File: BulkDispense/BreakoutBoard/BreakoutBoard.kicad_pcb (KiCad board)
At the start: 2 copper layers, 74.5 x 119 mm, 36 parts, among them J1 BS1, J10 OS3, J11 OS4, J12 FS1, J13 FS3, J14 PCV, J15 FS2, J16 FS4, J17 WL1, J18 WL2, J19 Analog Inputs, J2 BS2, J20 R0~R3, J21 R4~R7, J22 R8~R9, J23 Digital IN + R0~R4, J24 WB1, J25 WB2, J26 Digital Outputs, J27 R4~R9, J28 WV1, J29 WV2, J3 OS1, J30 Flow Sensors (PORT2), J4 OS2, J5 PS, J6 MV1&2, J7 MV3&4, J8 BS3, J9 BS4

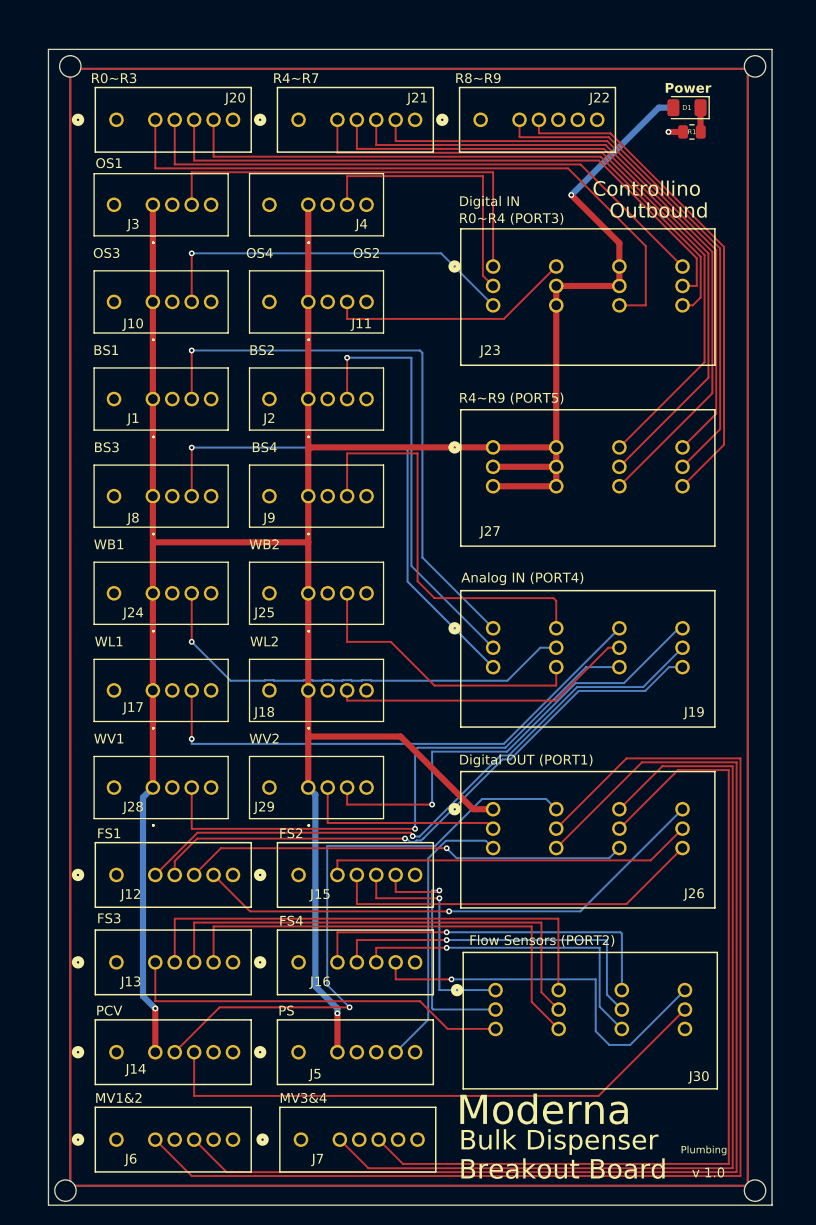
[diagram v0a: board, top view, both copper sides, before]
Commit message: Design Overhaul
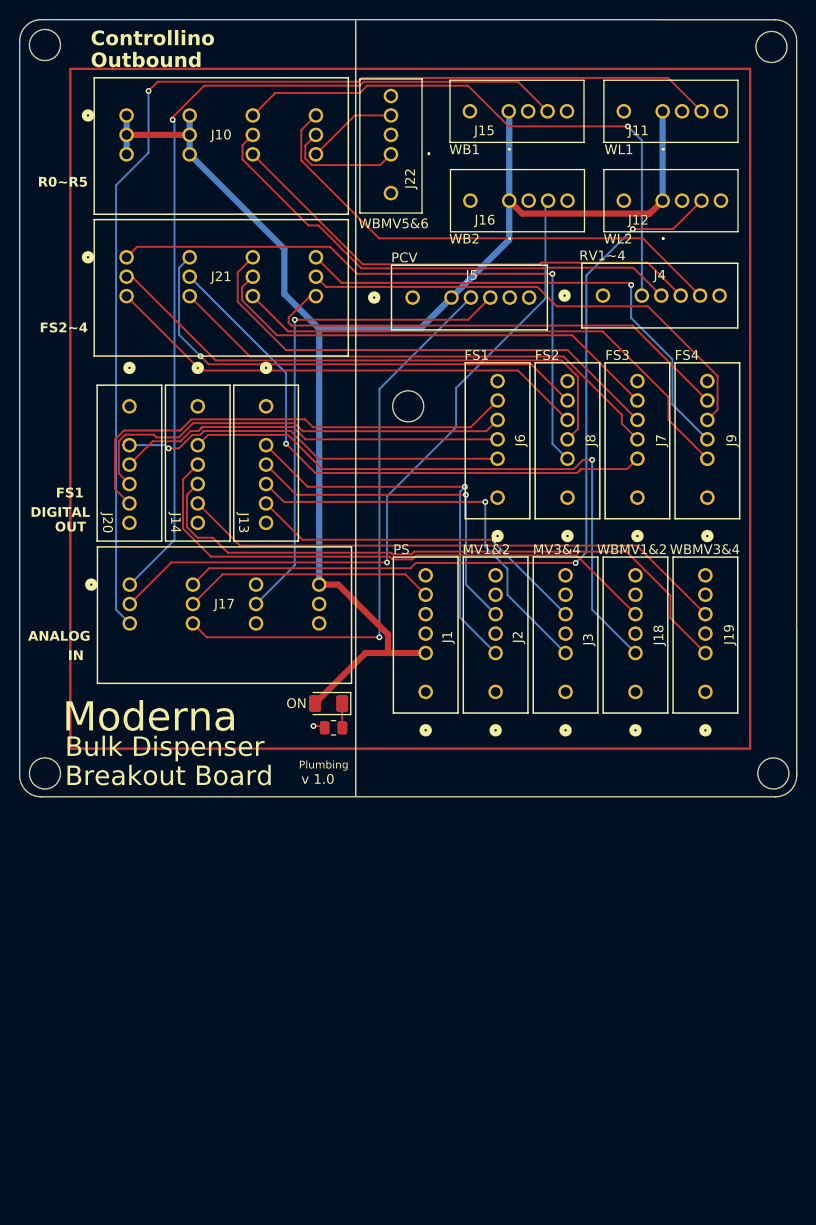
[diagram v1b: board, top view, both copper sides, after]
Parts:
- removed J23: Digital IN + R0~R4, PartsLibrary:CONN_37212-62M3-003PL_3MM
- removed J24: WB1, PartsLibrary:3720362A3003PL
- removed J25: WB2, PartsLibrary:3720362A3003PL
- removed J26: Digital Outputs, PartsLibrary:CONN_37212-62M3-003PL_3MM
- removed J27: R4~R9, PartsLibrary:CONN_37212-62M3-003PL_3MM
- removed J28: WV1, PartsLibrary:3720362A3003PL
- removed J29: WV2, PartsLibrary:3720362A3003PL
- removed J30: Flow Sensors (PORT2), PartsLibrary:CONN_37212-62M3-003PL_3MM
- added H5: MountingHole, MountingHole:MountingHole_3.2mm_M3, F.Cu at (181.8, 106.8)
- H1, H2, H3, H4: footprint MountingHole:MountingHole_2.2mm_M2 -> MountingHole:MountingHole_3.2mm_M3
- J1: value BS1 -> PS; footprint PartsLibrary:3720362A3003PL -> PartsLibrary:CONN_37204-62A3-004PL_3MM
- J10: value OS3 -> R0~R5; footprint PartsLibrary:3720362A3003PL -> PartsLibrary:CONN_37212-62M3-003PL_3MM
- J11: value OS4 -> WL1
- J12: value FS1 -> WL2; footprint PartsLibrary:CONN_37204-62A3-004PL_3MM -> PartsLibrary:3720362A3003PL
- J13: value FS3 -> DigitalOUT 0~3
- J14: value PCV -> DigitalOUT 4~7
- J15: value FS2 -> WB1; footprint PartsLibrary:CONN_37204-62A3-004PL_3MM -> PartsLibrary:3720362A3003PL
- J16: value FS4 -> WB2; footprint PartsLibrary:CONN_37204-62A3-004PL_3MM -> PartsLibrary:3720362A3003PL
- J17: value WL1 -> AnalogIOs; footprint PartsLibrary:3720362A3003PL -> PartsLibrary:CONN_37212-62M3-003PL_3MM
- J18: value WL2 -> WBMV1&2; footprint PartsLibrary:3720362A3003PL -> PartsLibrary:CONN_37204-62A3-004PL_3MM
- J19: value Analog Inputs -> WBMV3&4; footprint PartsLibrary:CONN_37212-62M3-003PL_3MM -> PartsLibrary:CONN_37204-62A3-004PL_3MM
- J2: value BS2 -> MV1&2; footprint PartsLibrary:3720362A3003PL -> PartsLibrary:CONN_37204-62A3-004PL_3MM
- J20: value R0~R3 -> FS1
- J21: value R4~R7 -> FS2~FS4; footprint PartsLibrary:CONN_37204-62A3-004PL_3MM -> PartsLibrary:CONN_37212-62M3-003PL_3MM
- J22: value R8~R9 -> WB-MV5&6; footprint PartsLibrary:CONN_37204-62A3-004PL_3MM -> PartsLibrary:3720362A3003PL
- J3: value OS1 -> MV3&4; footprint PartsLibrary:3720362A3003PL -> PartsLibrary:CONN_37204-62A3-004PL_3MM
- J4: value OS2 -> RV1~4; footprint PartsLibrary:3720362A3003PL -> PartsLibrary:CONN_37204-62A3-004PL_3MM
- J5: value PS -> PCV
- J6: value MV1&2 -> FS1
- J7: value MV3&4 -> FS3
- J8: value BS3 -> FS2; footprint PartsLibrary:3720362A3003PL -> PartsLibrary:CONN_37204-62A3-004PL_3MM
- J9: value BS4 -> FS4; footprint PartsLibrary:3720362A3003PL -> PartsLibrary:CONN_37204-62A3-004PL_3MM
- moved H3 138.4 mm to (181.6, 32.0)
- moved J12 86.9 mm to (170.4, 47.8)
- moved H4 84.8 mm to (106.8, 106.8)
- moved J15 80.6 mm to (154.6, 38.6)
- moved J16 80.4 mm to (154.6, 47.8)
- moved J5 78.6 mm to (148.7, 57.8)
- moved J6 78.5 mm to (153.4, 74.4), turned to 90 degrees
- moved J7 76.5 mm to (167.8, 74.4), turned to 90 degrees
- moved H2 73.1 mm to (106.8, 31.8)
- moved D1 71.6 mm to (136.0, 99.6)
- moved R1 71.6 mm to (136.5, 102.1)
- moved J3 62.7 mm to (160.4, 94.4), turned to 90 degrees
- moved J14 62.7 mm to (122.5, 73.0), turned to -90 degrees
- moved J13 54.5 mm to (129.6, 73.0), turned to -90 degrees
- moved H1 49.3 mm to (144.2, 69.0)
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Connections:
- J1 pad 3: /AI0 -> GND
- J10 pad 2: GND -> +24V
- J10 pad 3: /DI2 -> +24V
- J11 pad 3: /DI3 -> /AI6
- J12 pad 1: /FS1-1 -> +24V
- J12 pad 2: /FS1-2 -> GND
- J12 pad 3: /FS1-3 -> /AI7
- J13 pad 1: /FS3-1 -> /DO0
- J13 pad 2: /FS3-2 -> /DO1
- J13 pad 3: /FS3-3 -> /DO2
- J13 pad 4: /FS3-4 -> /DO3
- J14 pad 1: +24V -> /DO4
- J14 pad 2: /AI13 -> /DO5
- J14 pad 3: /AO0 -> /DO6
- J14 pad 4: GND -> /DO7
- J15 pad 1: /FS2-1 -> +24V
- J15 pad 2: /FS2-2 -> GND
- J15 pad 3: /FS2-3 -> /AI4
- J16 pad 1: /FS4-1 -> +24V
- J16 pad 2: /FS4-2 -> GND
- J16 pad 3: /FS4-3 -> /AI5
- J17 pad 1: +24V -> /AI4
- J17 pad 2: GND -> /AI5
- J18 pad 1: +24V -> /DO4
- J18 pad 3: /AI7 -> /DO5
- J19 pad 1: /AI0 -> /DO6
- J19 pad 2: /AI1 -> GND
- J19 pad 3: /AI2 -> /DO7
- J19 pad 4: /AI3 -> GND
- J19 pad 5: /AI4 -> (no net)
- J19 pad 6: /AI5 -> (no net)
- J2 pad 1: +24V -> /DO0
- J2 pad 3: /AI1 -> /DO1
- J20 pad 1: /R0_OUT -> /FS1-1
- J20 pad 2: /R1_OUT -> /FS1-2
- J20 pad 3: /R2_OUT -> /FS1-3
- J20 pad 4: /R3_OUT -> /FS1-4
- J21 pad 1: /R4_OUT -> /FS2-1
- J21 pad 2: /R5_OUT -> /FS2-2
- J21 pad 3: /R6_OUT -> /FS2-3
- J21 pad 4: /R7_OUT -> /FS2-4
- J21 pad 5: (no net) -> /FS3-1
- J21 pad 6: (no net) -> /FS3-2
- J22 pad 1: /R8_OUT -> /R4_OUT
- J22 pad 2: /R9_OUT -> unconnected-(J22-Pin_2-Pad2)
- J22 pad 3: GND -> /R5_OUT
- J3 pad 1: +24V -> /DO2
- J3 pad 3: /DI0 -> /DO3
- J4 pad 1: +24V -> /R0_OUT
- J4 pad 2: GND -> /R1_OUT
- J4 pad 3: /DI1 -> /R2_OUT
- J5 pad 2: GND -> /AI13
- J5 pad 3: GND -> /AO0
- J5 pad 4: /AI12 -> GND
- J6 pad 1: /DO0 -> /FS1-1
- J6 pad 2: GND -> /FS1-2
- J6 pad 3: /DO1 -> /FS1-3
- J6 pad 4: GND -> /FS1-4
- J7 pad 1: /DO2 -> /FS3-1
- J7 pad 2: GND -> /FS3-2
- J7 pad 3: /DO3 -> /FS3-3
- J7 pad 4: GND -> /FS3-4
- J8 pad 1: +24V -> /FS2-1
- J8 pad 2: GND -> /FS2-2
- J8 pad 3: /AI2 -> /FS2-3
- J9 pad 1: +24V -> /FS4-1
- J9 pad 2: GND -> /FS4-2
- J9 pad 3: /AI3 -> /FS4-3
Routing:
- net +24V: track 306.2 -> 151.7 mm, vias 3 -> 0
- net /DO1: track 121.7 -> 35.4 mm, vias 0 -> 1
- net /DO0: track 126.8 -> 41.1 mm, vias 0 -> 1
- net /R6_OUT: track 69.9 -> 0.00 mm
- net /DO6: track 0.00 -> 65.3 mm
- net /DO4: track 0.00 -> 64.6 mm, vias 0 -> 1
- net /R7_OUT: track 61.6 -> 0.00 mm
- net /AI6: track 54.5 -> 115.9 mm
- net /AI0: track 60.2 -> 0.00 mm, vias 1 -> 0
- net /R5_OUT: track 69.4 -> 9.38 mm
- net /AI8: track 59.9 -> 0.00 mm, vias 1 -> 0
- net /DO5: track 0.00 -> 58.0 mm
- net /DO7: track 0.00 -> 57.0 mm
- net /R4_OUT: track 69.0 -> 12.5 mm
- net /DO3: track 91.4 -> 35.8 mm, vias 0 -> 1
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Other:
- board size 74.5 x 119 mm -> 80 x 80 mm
- board text added: "ANALOG"
- board text added: "DIGITAL"
- board text added: "FS1"
- board text added: "FS2~4"
- board text added: "IN"
- board text added: "ON"
- board text added: "OUT"
- board text added: "R0~R5"
- board text added: "WB1"
- board text added: "WB2"
- board text added: "WBMV5&6"
- board text added: "WL1"
- board text added: "WL2"
- board text removed: "Analog IN (PORT4)"
- board text removed: "Digital IN"
- board text removed: "Digital OUT (PORT1)"
- board text removed: "Power"
- board text removed: "R0~R4 (PORT3)"
- board text removed: "R4~R9 (PORT5)"
